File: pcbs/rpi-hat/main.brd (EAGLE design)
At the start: 85.1 x 55.9 mm, 18 parts, among them IC1 MCP23017SP2, U1 MCP3002-I/P

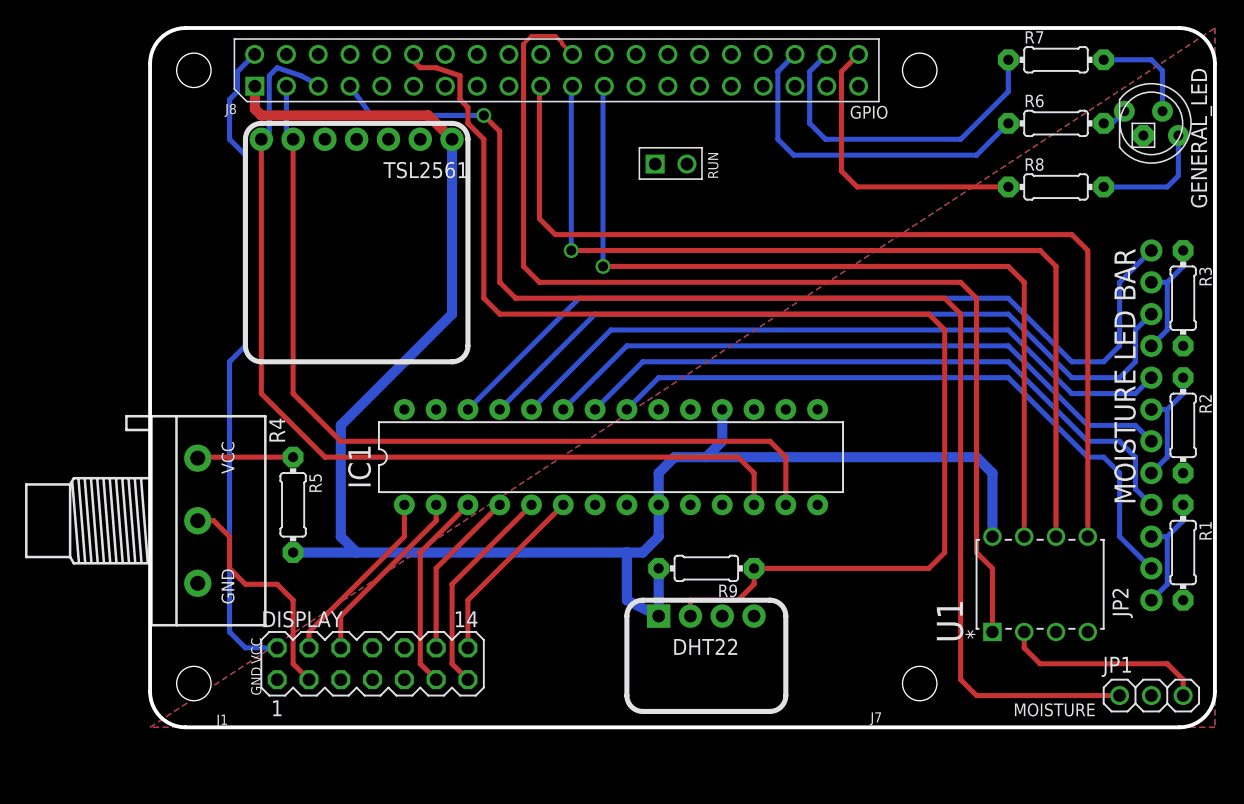
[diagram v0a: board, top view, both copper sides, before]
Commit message: chg
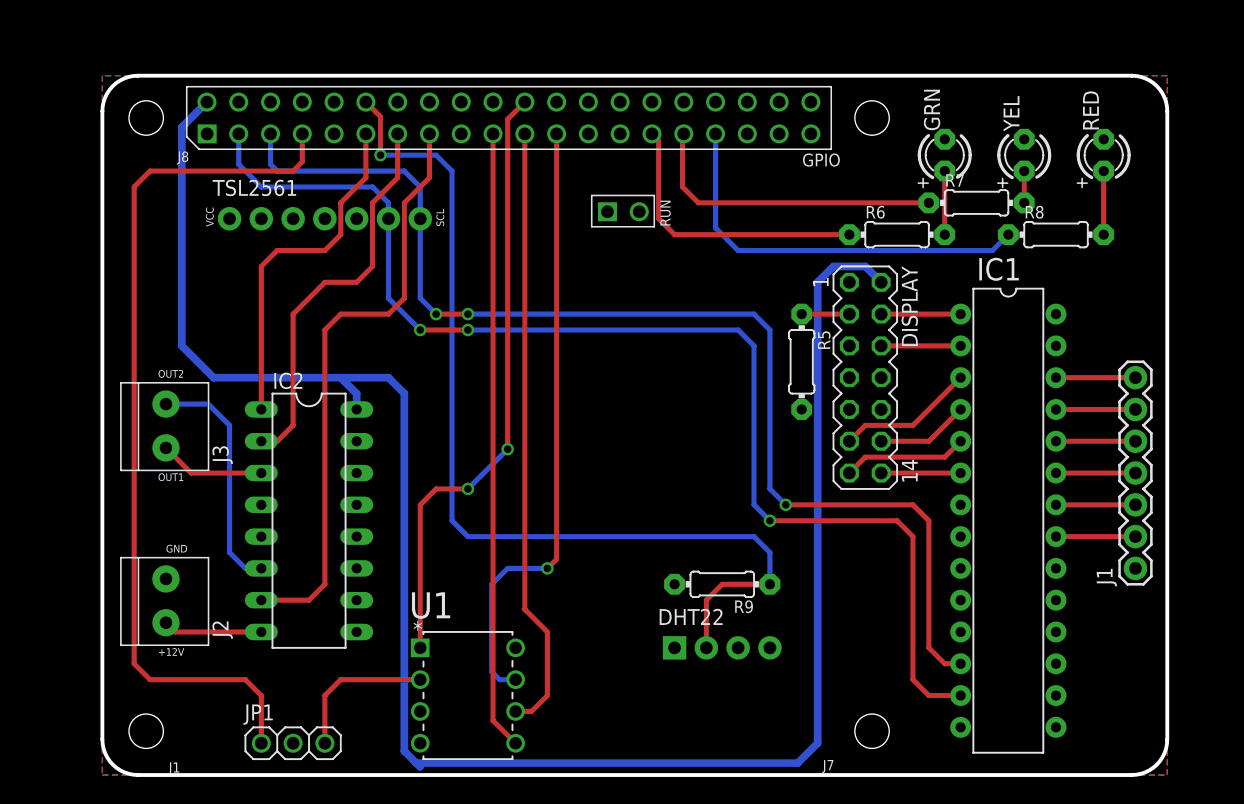
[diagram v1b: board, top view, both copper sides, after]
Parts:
- removed GENERAL_LED: RGBLED_CA-5MM, adafruit:LED5MMRGB
- removed JP2: (no value), adafruit:1X12-CB
- removed R1, R2, R3: 47, adafruit:0204/7
- removed R4: (no value), pot:3RP/1610N
- added GRN, RED, YEL: (no value), adafruit:LED3MM
- added IC2: L293D, st-microelectronics:DIL16
- added J1: (no value), SparkFun-Connectors:1X07
- added J2, J3: 1X2-3.5MM, adafruit:1X2-3.5MM
- moved JP1 68.7 mm to (15.2, 2.54)
- moved U1 48.6 mm to (33.0, 2.54), turned to 0 degrees
- moved DISPLAY 45.5 mm to (61.0, 31.8), turned to 270 degrees
- moved R5 42.2 mm to (55.9, 33.0)
- moved IC1 32.2 mm to (72.4, 20.3), turned to 270 degrees
- moved TSL2561 18.9 mm to (10.2, 44.5), turned to 0 degrees
- moved R6 15.5 mm to (63.5, 43.2)
- moved R7 13.1 mm to (69.8, 45.7)
- moved PCB1 5.39 mm to (0.00, 0.00)
- moved R8 3.81 mm to (76.2, 43.2)
- moved DHT22 2.84 mm to (45.7, 10.2)
- moved R9 1.80 mm to (49.5, 15.2)
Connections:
- net N$11 renamed MGPB0
- net N$13 renamed MGPB1
- net N$14 renamed MGPB2
- net N$15 renamed MGPB3
- net N$16 renamed MGPB4
- net N$17 renamed MGPB5
- removed net BAR_3: IC1.23, JP2.6
- removed net BAR_4: IC1.24, JP2.8
- removed net BAR_5: IC1.25, JP2.10
- removed net BAR_6: IC1.26, JP2.12
- removed net BAR_R: IC1.22, JP2.4
- removed net BAR_T: IC1.21, JP2.2
- removed net GBLUE: PCB1.P$40, R8.1
- removed net GGRN: PCB1.P$38, R7.1
- removed net GRED: PCB1.P$36, R6.1
- removed net N$10: JP2.11, JP2.9, R3.1
- removed net N$12: R4.1, R5.1
- removed net N$9: JP2.5, JP2.7, R2.1
- removed net POT: DISPLAY.3, R4.2
- new net +12V: IC2.8, J2.1
- new net GND3: IC2.13
- new net GND4: IC2.12
- new net GPIO13: PCB1.P$33, R8.1
- new net GPIO22: IC2.7, PCB1.P$15
- new net GPIO27: IC2.2, PCB1.P$13
- new net GPIO5: PCB1.P$29, R6.1
- new net GPIO6: PCB1.P$31, R7.1
- new net N$1: IC1.26, J1.7
- new net N$2: IC1.25, J1.6
- new net N$3: IC1.24, J1.5
- new net N$4: IC1.23, J1.4
- new net N$5: IC1.22, J1.3
- new net N$7: IC1.21, J1.2
- new net OUT1: IC2.3, J3.1
- new net OUT2: IC2.6, J3.2
- new net PWM1: IC2.1, PCB1.P$11
- net 5V: now also IC2.16
- net GND: now also GRN.K, IC2.4, IC2.5, J1.1, J2.2, RED.K, YEL.K; no longer GENERAL_LED.2, R1.2, R2.2, R3.2, R4.3
- net N$18: now also GRN.A; no longer GENERAL_LED.1
- net N$19: now also YEL.A; no longer GENERAL_LED.3
- net N$20: now also RED.A; no longer GENERAL_LED.4
- net N$8: now also DISPLAY.3, R5.1; no longer JP2.1, JP2.3, R1.1
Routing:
- net VCC: track 138.2 -> 0.00 mm
- net 5V: track 52.4 -> 148.8 mm
- net BAR_6: track 67.1 -> 0.00 mm
- net BAR_5: track 60.9 -> 0.00 mm
- net BAR_4: track 54.8 -> 0.00 mm
- net BAR_T: track 52.3 -> 0.00 mm
- net BAR_R: track 52.3 -> 0.00 mm
- net BAR_3: track 52.3 -> 0.00 mm
- net GPIO22: track 0.00 -> 47.3 mm
- net CE0: track 87.1 -> 48.6 mm, vias 0 -> 2
- net GPIO4: track 106.1 -> 69.6 mm, vias 1 -> 0
- net GPIO13: track 0.00 -> 32.2 mm
- net GPIO27: track 0.00 -> 31.3 mm
- net MOSI: track 78.4 -> 49.4 mm
- net PWM1: track 0.00 -> 27.7 mm
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- added copper zone on layer 1, net VCC
- removed copper zone on layer 1, net GND
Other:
- board text added: "+12V"
- board text added: "OUT1"
- board text added: "OUT2"
- board text added: "SCL"
- board text removed: "MOISTURE"
- board text removed: "MOISTURE LED BAR"
